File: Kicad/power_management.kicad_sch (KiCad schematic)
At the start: 32 parts, among them U3 BQ25896RTWR, U4 BQ27220YZFR

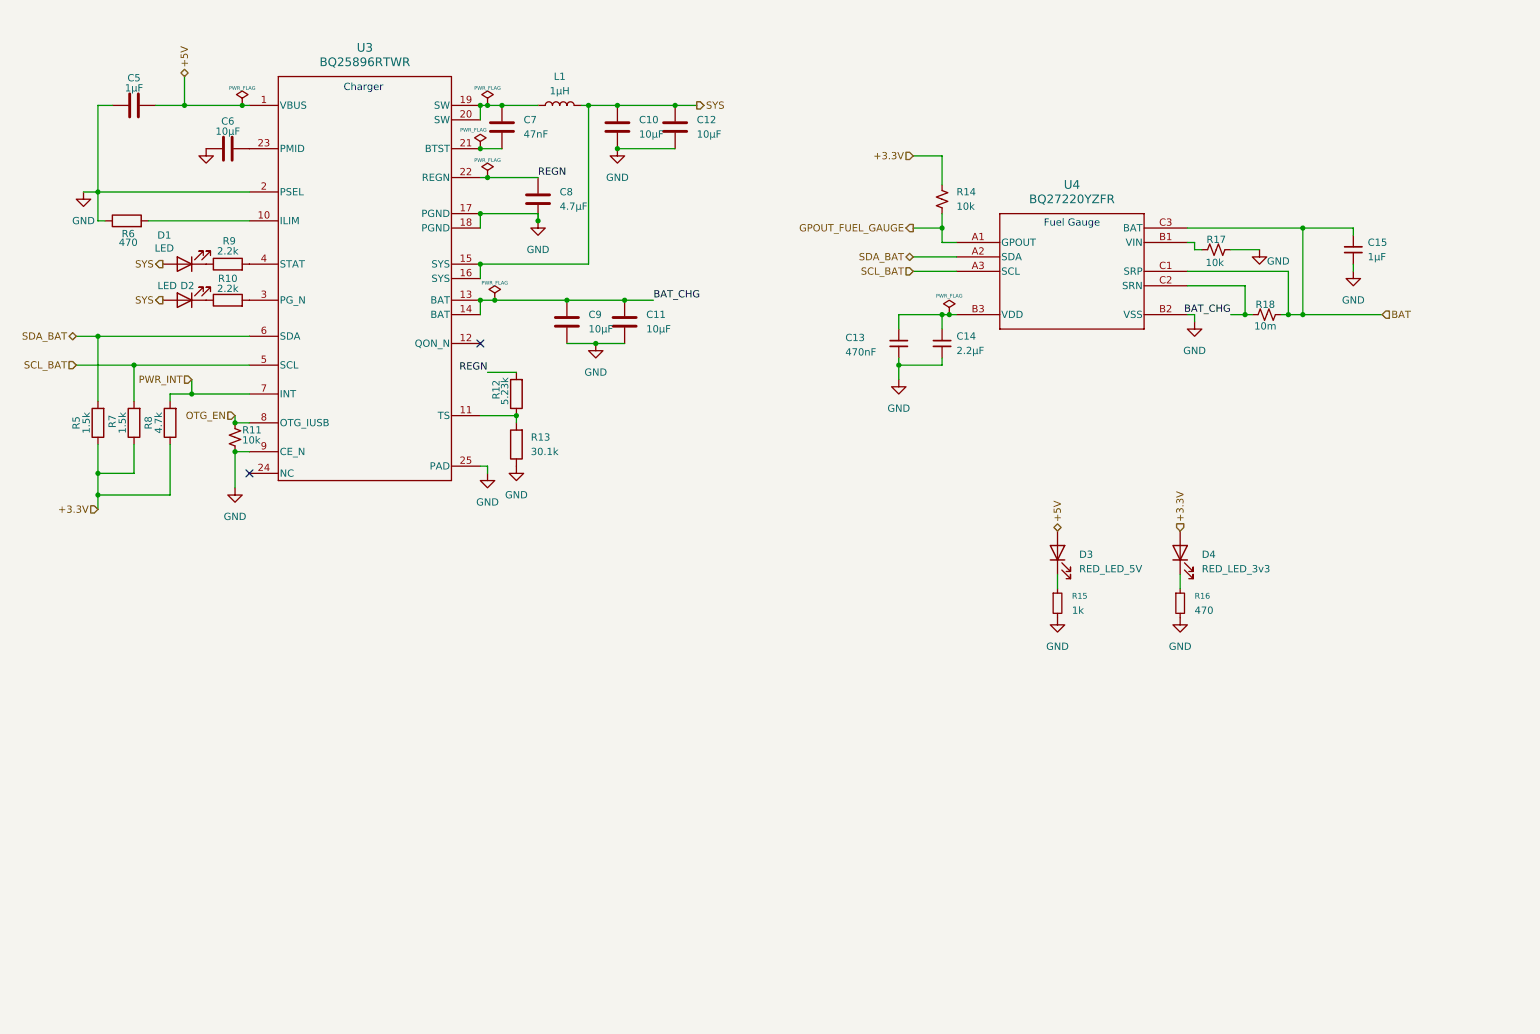
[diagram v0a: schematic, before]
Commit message: feat: electrical schematic validated
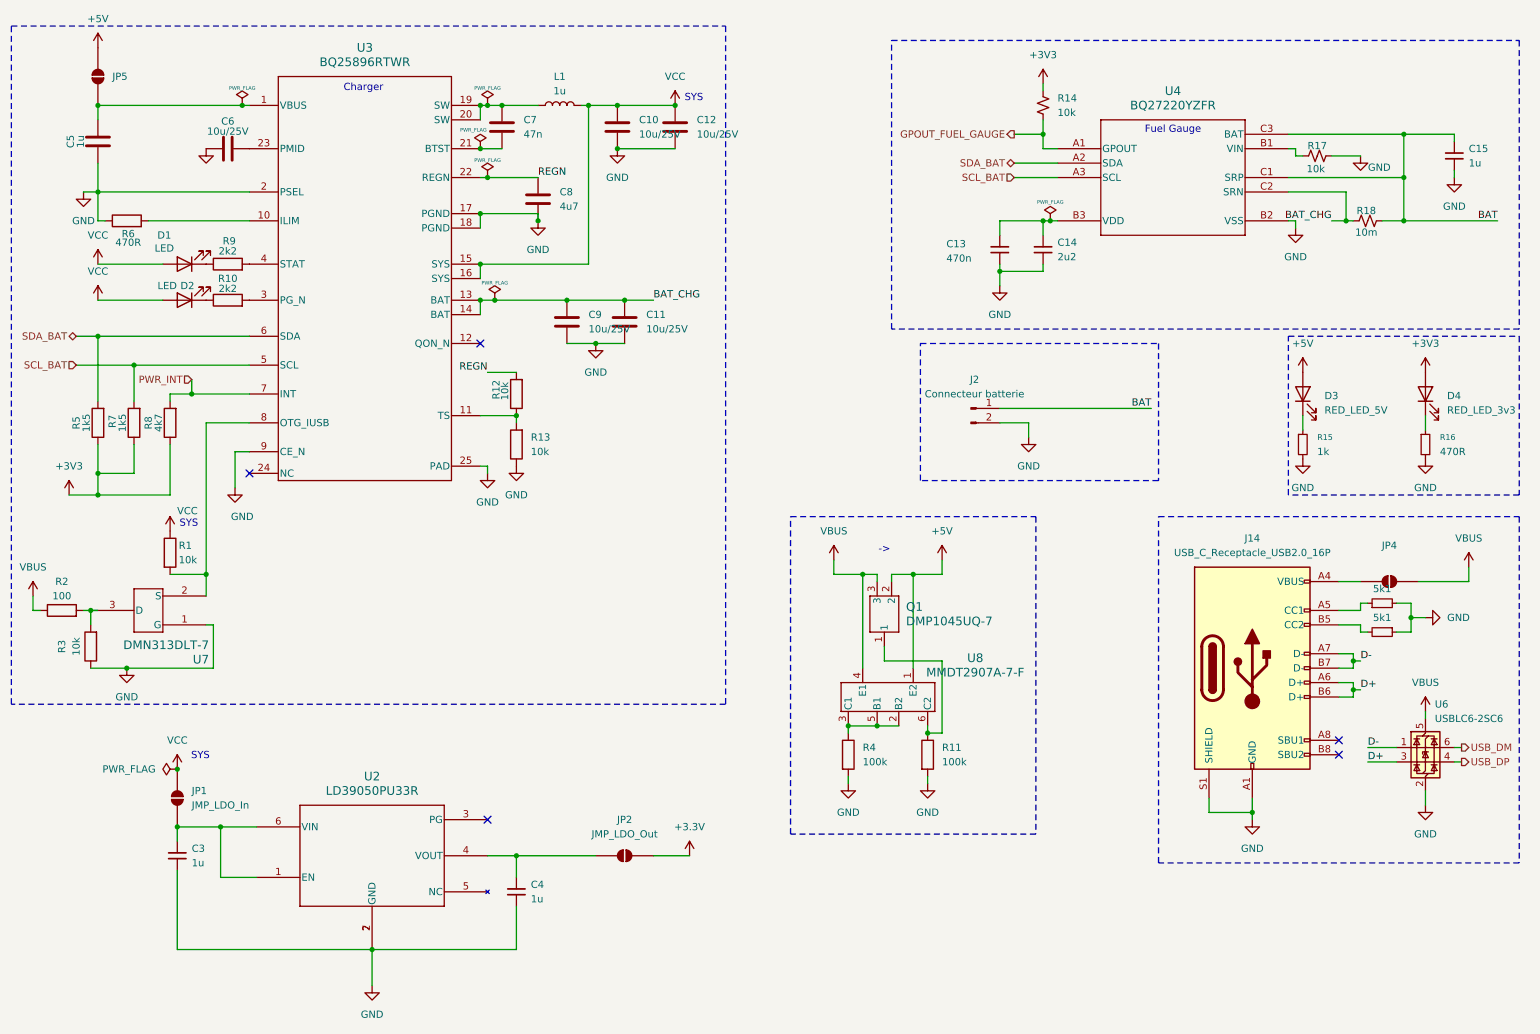
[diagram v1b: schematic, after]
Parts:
- removed R11: 10k, Resistor_SMD:R_0402_1005Metric, symbol Device:R_Small_US
- added C3, C4: 1u, Capacitor_SMD:C_0402_1005Metric, symbol Device:C_Small
- added J14: USB_C_Receptacle_USB2.0_16P, Connector_USB:USB_C_Receptacle_GCT_USB4105-xx-A_16P_TopMnt_Horizontal, symbol Connector:USB_C_Receptacle_USB2.0_16P
- added J2: Connecteur batterie, Connector_JST:JST_XH_B2B-XH-A_1x02_P2.50mm_Vertical, symbol Connector:Conn_01x02_Pin
- added JP1: JMP_LDO_In, Jumper:SolderJumper-2_P1.3mm_Open_TrianglePad1.0x1.5mm, symbol Jumper:SolderJumper_2_Open
- added JP2: JMP_LDO_Out, Jumper:SolderJumper-2_P1.3mm_Open_TrianglePad1.0x1.5mm, symbol Jumper:SolderJumper_2_Open
- added JP4, JP5: JMP_Battery, Jumper:SolderJumper-2_P1.3mm_Open_TrianglePad1.0x1.5mm, symbol Jumper:SolderJumper_2_Open
- added Q1: DMP1045UQ-7, DMP1045UQ-7_DIO, symbol DMP1045UQ-7:DMP1045UQ-7
- added R1, R3: 10k, Resistor_SMD:R_0402_1005Metric, symbol Device:R
- added R11, R4: 100k, Resistor_SMD:R_0402_1005Metric, symbol Device:R
- added R2: 100, Resistor_SMD:R_0402_1005Metric, symbol Device:R
- added R20, R21: 5k1, Resistor_SMD:R_0402_1005Metric, symbol Device:R_Small
- added U2: LD39050PU33R, footprints_LD39:DFN6_3X3_STM, symbol LD39050PU33R:LD39050PU33R
- added U6: USBLC6-2SC6, Package_TO_SOT_SMD:SOT-23-6, symbol Power_Protection:USBLC6-2SC6
- added U7: DMN313DLT-7, SOT-523_DIO, symbol DMN313DLT:DMN313DLT-7
- added U8: MMDT2907A-7-F, SOT-363_DIO, symbol MMDT2907A-7-F:MMDT2907A-7-F
- C10, C11, C12, C6, C9: value 10µF -> 10u/25V
- C13: value 470nF -> 470n; footprint Capacitor_SMD:C_0603_1608Metric -> Capacitor_SMD:C_0402_1005Metric
- C14: value 2.2µF -> 2u2; footprint Capacitor_SMD:C_0603_1608Metric -> Capacitor_SMD:C_0402_1005Metric
- C15, C5: value 1µF -> 1u
- C7: value 47nF -> 47n; footprint Capacitor_SMD:C_0603_1608Metric -> Capacitor_SMD:C_0402_1005Metric
- C8: value 4.7µF -> 4u7
- D3, D4: footprint LED_SMD:LED_Cree-XHP50_3V_HighDensity -> LED_SMD:LED_0603_1608Metric
- L1: value 1µH -> 1u
- R10, R9: value 2.2k -> 2k2
- R12: value 5.23k -> 10k
- R13: value 30.1k -> 10k
- R16, R6: value 470 -> 470R
- R5, R7: value 1.5k -> 1k5
- R8: value 4.7k -> 4k7
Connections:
- net +3.3V: now also JP2.2 (B); no longer D4.2 (A), R14.1, R5.1, R7.1, R8.1
- net +5V: now also JP5.2 (B), Q1.2, U8.1 (E2); no longer C5.2, U3.1 (VBUS)
- net BAT: now also J2.1 (Pin_1)
- net GND: now also C3.2, C4.2, J14.A1 (GND), J14.A12 (GND), J14.B1 (GND), J14.B12 (GND), J14.S1 (SHIELD), J2.2 (Pin_2), R11.2, R20.2, R21.1, R3.1, R4.2, U2.2 (GND), U2.7 (GND), U6.2 (GND), U7.1 (G)
- net OTG_EN: no longer names the net of U3.8 (OTG_IUSB)
- net OTG_EN: now also R1.2, U7.2 (S)
- net SYS renamed VCC
- net VCC: now also JP1.2 (B), R1.1
- new net: C5.2, JP5.1 (A), U3.1 (VBUS)
- new net: C3.1, JP1.1 (A), U2.1 (EN), U2.6 (VIN)
- new net: C4.1, JP2.1 (A), U2.4 (VOUT)
- new net: R2.2, R3.2, U7.3 (D)
- new net: J14.A4 (VBUS), J14.A9 (VBUS), J14.B4 (VBUS), J14.B9 (VBUS), JP4.1 (A)
- new net: Q1.1, R11.1, U8.6 (C2)
- new net: J14.B5 (CC2), R21.2
- new net: J14.A5 (CC1), R20.1
- new net: R4.1, U8.2 (B2), U8.3 (C1), U8.5 (B1)
- new net +3V3: D4.2 (A), R14.1, R5.1, R7.1, R8.1
- new net D+: J14.A6 (D+), J14.B6 (D+), U6.3 (I/O2)
- new net D-: J14.A7 (D-), J14.B7 (D-), U6.1 (I/O1)
- new net USB_DM: U6.6 (I/O1)
- new net USB_DP: U6.4 (I/O2)
- new net VBUS: JP4.2 (B), Q1.3, R2.1, U6.5 (VBUS), U8.4 (E1)
- no-connect marks 2 -> 5
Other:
- note added: "->"
- note added: "SYS"
- moved on the sheet: C13, C14, C15, C5, D3, D4, R14, R15, R16, R17, R18, U4
